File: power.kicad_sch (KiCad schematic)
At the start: 12 parts, among them U4 L78L05_SOT89, U4 MIC2288

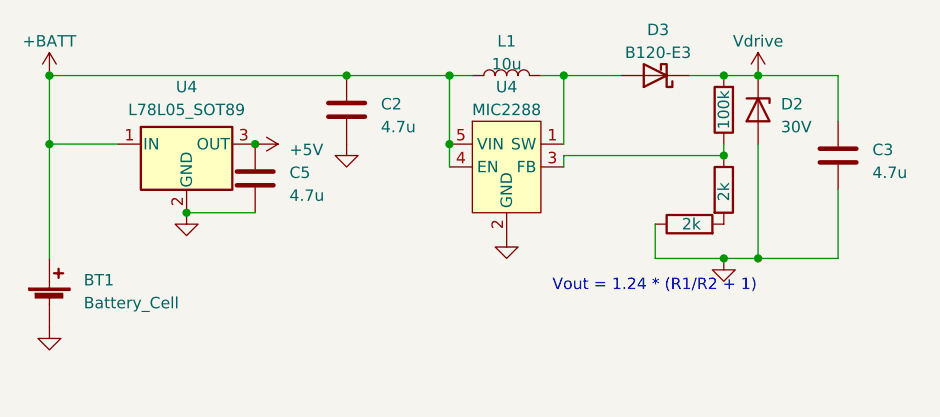
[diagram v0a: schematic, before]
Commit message: Work
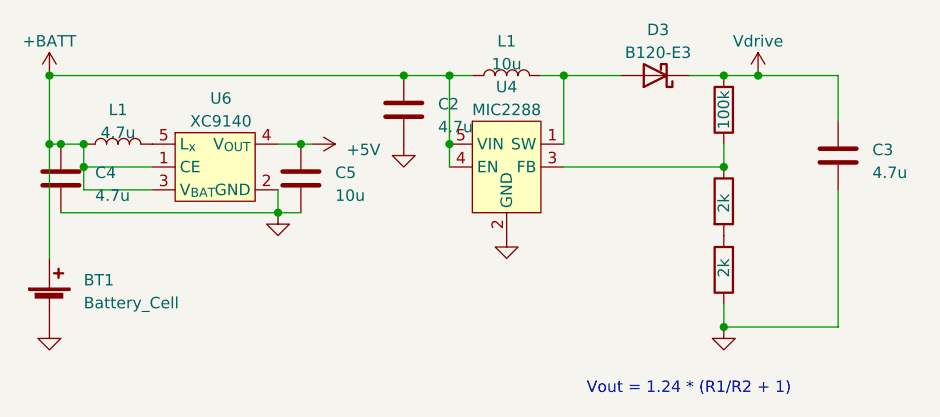
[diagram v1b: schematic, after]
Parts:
- removed D2: 30V, Diode_SMD:D_SOD-123, symbol Device:D_Zener
- removed U4: L78L05_SOT89, Package_TO_SOT_SMD:TO-252-2, symbol Regulator_Linear:L78L05_SOT89
- added C4: 4.7u, Capacitor_SMD:C_1206_3216Metric_Pad1.33x1.80mm_HandSolder, symbol Device:C
- added L1: 4.7u, Inductor_SMD:L_Coilcraft_XAL4030-XXX, symbol Device:L
- added U6: XC9140, Package_SO:TSOP-5_1.65x3.05mm_P0.95mm, symbol custom_symbols:XC9140
- C5: value 4.7u -> 10u
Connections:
- net +5V: now also U6.4 (V_{OUT})
- net +BATT: now also C4.1, L1.1, U6.1 (CE), U6.3 (V_{BAT})
- net GND: now also C4.2, U6.2 (GND)
- new net: L1.2, U6.5 (L_{x})
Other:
- moved on the sheet: C2, C5
